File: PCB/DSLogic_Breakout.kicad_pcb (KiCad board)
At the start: 2 copper layers, 24 x 74 mm, 5 parts, among them J1 Interconnect

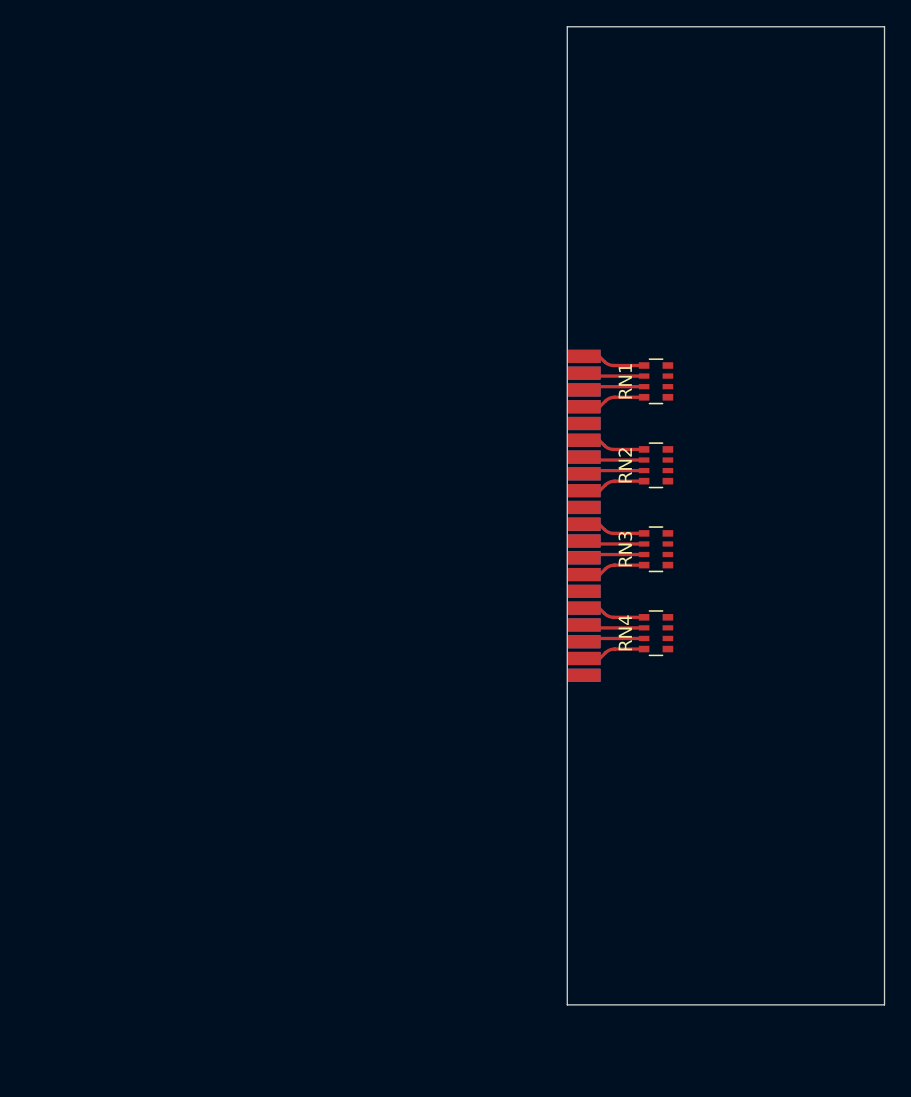
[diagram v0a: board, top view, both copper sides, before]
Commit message: Rev 1 Done
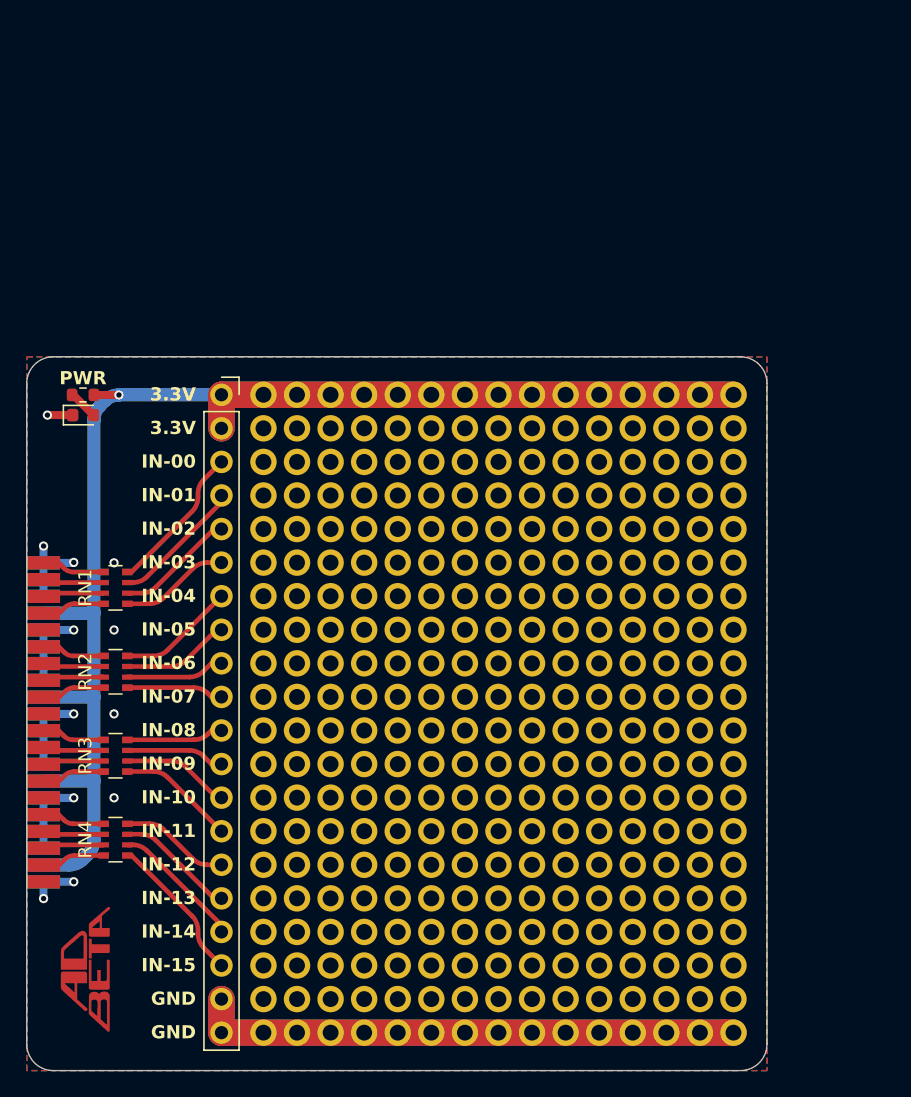
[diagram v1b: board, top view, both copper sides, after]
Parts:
- added ?: , , F.Cu at (141.1, 102.9)
- added ?: , , F.Cu at (123.3, 102.9)
- added ?: , , F.Cu at (125.9, 102.9)
- added ?: , , F.Cu at (133.5, 102.9)
- added ?: , , F.Cu at (141.1, 54.6)
- added ?: , , F.Cu at (133.5, 54.6)
- added ?: , , F.Cu at (151.3, 102.9)
- added ?: , , F.Cu at (146.2, 54.6)
- added ?: , , F.Cu at (156.3, 54.6)
- added ?: , , F.Cu at (138.6, 54.6)
- added ?: , , F.Cu at (136.0, 54.6)
- added ?: , , F.Cu at (151.3, 54.6)
- added ?: , , F.Cu at (123.3, 54.6)
- added ?: , , F.Cu at (146.2, 102.9)
- added ?: , , F.Cu at (148.7, 54.6)
- added ?: , , F.Cu at (153.8, 102.9)
- added ?: , , F.Cu at (130.9, 102.9)
- added ?: , , F.Cu at (130.9, 54.6)
- added ?: , , F.Cu at (120.8, 102.9)
- added ?: , , F.Cu at (128.4, 54.6)
- added ?: , , F.Cu at (156.3, 102.9)
- added ?: , , F.Cu at (128.4, 102.9)
- added ?: , , F.Cu at (148.7, 102.9)
- added ?: , , F.Cu at (143.6, 54.6)
- added ?: , , F.Cu at (153.8, 54.6)
- added ?: , , F.Cu at (138.6, 102.9)
- added ?: , , F.Cu at (143.6, 102.9)
- added ?: , , F.Cu at (136.0, 102.9)
- added ?: , , F.Cu at (125.9, 54.6)
- added D1: PWR, LED_SMD:LED_0603_1608Metric, F.Cu at (107.1, 56.1)
- added J2: Conn_Input, Connector_PinSocket_2.54mm:PinSocket_1x20_P2.54mm_Vertical, F.Cu at (117.6, 54.6)
- added R1: 2K2, Resistor_SMD:R_0603_1608Metric, F.Cu at (107.1, 54.6)
- added REF**: Protoboard_Hole, Footprints:Protoboard_Hole, F.Cu at (125.9, 72.4)
- added REF**: Protoboard_Hole, Footprints:Protoboard_Hole, F.Cu at (156.3, 59.7)
- added REF**: Protoboard_Hole, Footprints:Protoboard_Hole, F.Cu at (128.4, 67.3)
- added REF**: Protoboard_Hole, Footprints:Protoboard_Hole, F.Cu at (125.9, 97.8)
- added REF**: Protoboard_Hole, Footprints:Protoboard_Hole, F.Cu at (128.4, 74.9)
- added REF**: Protoboard_Hole, Footprints:Protoboard_Hole, F.Cu at (156.3, 67.3)
- added REF**: Protoboard_Hole, Footprints:Protoboard_Hole, F.Cu at (141.1, 85.1)
- added REF**: Protoboard_Hole, Footprints:Protoboard_Hole, F.Cu at (133.5, 72.4)
- added REF**: Protoboard_Hole, Footprints:Protoboard_Hole, F.Cu at (141.1, 57.1)
- added REF**: Protoboard_Hole, Footprints:Protoboard_Hole, F.Cu at (123.3, 62.2)
- added REF**: Protoboard_Hole, Footprints:Protoboard_Hole, F.Cu at (141.1, 59.7)
- added REF**: Protoboard_Hole, Footprints:Protoboard_Hole, F.Cu at (128.4, 95.2)
- added REF**: Protoboard_Hole, Footprints:Protoboard_Hole, F.Cu at (146.2, 85.1)
- added REF**: Protoboard_Hole, Footprints:Protoboard_Hole, F.Cu at (156.3, 82.5)
- added REF**: Protoboard_Hole, Footprints:Protoboard_Hole, F.Cu at (120.8, 82.5)
- added REF**: Protoboard_Hole, Footprints:Protoboard_Hole, F.Cu at (148.7, 90.2)
- added REF**: Protoboard_Hole, Footprints:Protoboard_Hole, F.Cu at (146.2, 77.5)
- added REF**: Protoboard_Hole, Footprints:Protoboard_Hole, F.Cu at (151.3, 87.6)
- added REF**: Protoboard_Hole, Footprints:Protoboard_Hole, F.Cu at (151.3, 59.7)
- added REF**: Protoboard_Hole, Footprints:Protoboard_Hole, F.Cu at (143.6, 90.2)
- added REF**: Protoboard_Hole, Footprints:Protoboard_Hole, F.Cu at (153.8, 95.2)
- added REF**: Protoboard_Hole, Footprints:Protoboard_Hole, F.Cu at (138.6, 85.1)
- added REF**: Protoboard_Hole, Footprints:Protoboard_Hole, F.Cu at (125.9, 95.2)
- added REF**: Protoboard_Hole, Footprints:Protoboard_Hole, F.Cu at (125.9, 80.0)
- added REF**: Protoboard_Hole, Footprints:Protoboard_Hole, F.Cu at (143.6, 69.8)
- added REF**: Protoboard_Hole, Footprints:Protoboard_Hole, F.Cu at (123.3, 64.8)
- added REF**: Protoboard_Hole, Footprints:Protoboard_Hole, F.Cu at (128.4, 92.7)
- added REF**: Protoboard_Hole, Footprints:Protoboard_Hole, F.Cu at (156.3, 100.3)
- added REF**: Protoboard_Hole, Footprints:Protoboard_Hole, F.Cu at (136.0, 87.6)
- added REF**: Protoboard_Hole, Footprints:Protoboard_Hole, F.Cu at (123.3, 87.6)
- added REF**: Protoboard_Hole, Footprints:Protoboard_Hole, F.Cu at (156.3, 57.1)
- added REF**: Protoboard_Hole, Footprints:Protoboard_Hole, F.Cu at (156.3, 72.4)
- added REF**: Protoboard_Hole, Footprints:Protoboard_Hole, F.Cu at (151.3, 57.1)
- added REF**: Protoboard_Hole, Footprints:Protoboard_Hole, F.Cu at (133.5, 77.5)
- added REF**: Protoboard_Hole, Footprints:Protoboard_Hole, F.Cu at (153.8, 77.5)
- added REF**: Protoboard_Hole, Footprints:Protoboard_Hole, F.Cu at (120.8, 85.1)
- added REF**: Protoboard_Hole, Footprints:Protoboard_Hole, F.Cu at (123.3, 69.8)
- added REF**: Protoboard_Hole, Footprints:Protoboard_Hole, F.Cu at (146.2, 62.2)
- added REF**: Protoboard_Hole, Footprints:Protoboard_Hole, F.Cu at (128.4, 100.3)
- added REF**: Protoboard_Hole, Footprints:Protoboard_Hole, F.Cu at (151.3, 80.0)
- added REF**: Protoboard_Hole, Footprints:Protoboard_Hole, F.Cu at (130.9, 97.8)
- added REF**: Protoboard_Hole, Footprints:Protoboard_Hole, F.Cu at (130.9, 59.7)
- added REF**: Protoboard_Hole, Footprints:Protoboard_Hole, F.Cu at (130.9, 72.4)
- added REF**: Protoboard_Hole, Footprints:Protoboard_Hole, F.Cu at (141.1, 87.6)
- added REF**: Protoboard_Hole, Footprints:Protoboard_Hole, F.Cu at (120.8, 87.6)
- added REF**: Protoboard_Hole, Footprints:Protoboard_Hole, F.Cu at (141.1, 69.8)
- added REF**: Protoboard_Hole, Footprints:Protoboard_Hole, F.Cu at (148.7, 97.8)
- added REF**: Protoboard_Hole, Footprints:Protoboard_Hole, F.Cu at (130.9, 62.2)
- added REF**: Protoboard_Hole, Footprints:Protoboard_Hole, F.Cu at (141.1, 62.2)
- added REF**: Protoboard_Hole, Footprints:Protoboard_Hole, F.Cu at (133.5, 59.7)
- added REF**: Protoboard_Hole, Footprints:Protoboard_Hole, F.Cu at (138.6, 69.8)
- added REF**: Protoboard_Hole, Footprints:Protoboard_Hole, F.Cu at (130.9, 92.7)
- added REF**: Protoboard_Hole, Footprints:Protoboard_Hole, F.Cu at (148.7, 77.5)
- added REF**: Protoboard_Hole, Footprints:Protoboard_Hole, F.Cu at (125.9, 69.8)
- added REF**: Protoboard_Hole, Footprints:Protoboard_Hole, F.Cu at (120.8, 67.3)
- added REF**: Protoboard_Hole, Footprints:Protoboard_Hole, F.Cu at (120.8, 72.4)
- added REF**: Protoboard_Hole, Footprints:Protoboard_Hole, F.Cu at (156.3, 92.7)
- added REF**: Protoboard_Hole, Footprints:Protoboard_Hole, F.Cu at (148.7, 82.5)
- added REF**: Protoboard_Hole, Footprints:Protoboard_Hole, F.Cu at (133.5, 100.3)
- added REF**: Protoboard_Hole, Footprints:Protoboard_Hole, F.Cu at (120.8, 62.2)
- added REF**: Protoboard_Hole, Footprints:Protoboard_Hole, F.Cu at (148.7, 57.1)
- added REF**: Protoboard_Hole, Footprints:Protoboard_Hole, F.Cu at (153.8, 82.5)
- added REF**: Protoboard_Hole, Footprints:Protoboard_Hole, F.Cu at (153.8, 87.6)
- added REF**: Protoboard_Hole, Footprints:Protoboard_Hole, F.Cu at (125.9, 62.2)
- added REF**: Protoboard_Hole, Footprints:Protoboard_Hole, F.Cu at (120.8, 95.2)
- added REF**: Protoboard_Hole, Footprints:Protoboard_Hole, F.Cu at (136.0, 64.8)
- added REF**: Protoboard_Hole, Footprints:Protoboard_Hole, F.Cu at (130.9, 100.3)
- added REF**: Protoboard_Hole, Footprints:Protoboard_Hole, F.Cu at (130.9, 69.8)
- added REF**: Protoboard_Hole, Footprints:Protoboard_Hole, F.Cu at (123.3, 59.7)
- added REF**: Protoboard_Hole, Footprints:Protoboard_Hole, F.Cu at (128.4, 87.6)
- added REF**: Protoboard_Hole, Footprints:Protoboard_Hole, F.Cu at (148.7, 85.1)
- added REF**: Protoboard_Hole, Footprints:Protoboard_Hole, F.Cu at (143.6, 87.6)
- added REF**: Protoboard_Hole, Footprints:Protoboard_Hole, F.Cu at (148.7, 92.7)
- added REF**: Protoboard_Hole, Footprints:Protoboard_Hole, F.Cu at (123.3, 57.1)
- added REF**: Protoboard_Hole, Footprints:Protoboard_Hole, F.Cu at (153.8, 72.4)
- added REF**: Protoboard_Hole, Footprints:Protoboard_Hole, F.Cu at (130.9, 80.0)
- added REF**: Protoboard_Hole, Footprints:Protoboard_Hole, F.Cu at (123.3, 77.5)
- added REF**: Protoboard_Hole, Footprints:Protoboard_Hole, F.Cu at (141.1, 77.5)
- added REF**: Protoboard_Hole, Footprints:Protoboard_Hole, F.Cu at (146.2, 82.5)
- added REF**: Protoboard_Hole, Footprints:Protoboard_Hole, F.Cu at (153.8, 80.0)
- added REF**: Protoboard_Hole, Footprints:Protoboard_Hole, F.Cu at (146.2, 87.6)
- added REF**: Protoboard_Hole, Footprints:Protoboard_Hole, F.Cu at (153.8, 69.8)
- added REF**: Protoboard_Hole, Footprints:Protoboard_Hole, F.Cu at (136.0, 57.1)
- added REF**: Protoboard_Hole, Footprints:Protoboard_Hole, F.Cu at (143.6, 72.4)
- added REF**: Protoboard_Hole, Footprints:Protoboard_Hole, F.Cu at (123.3, 72.4)
- added REF**: Protoboard_Hole, Footprints:Protoboard_Hole, F.Cu at (146.2, 74.9)
- added REF**: Protoboard_Hole, Footprints:Protoboard_Hole, F.Cu at (120.8, 74.9)
- added REF**: Protoboard_Hole, Footprints:Protoboard_Hole, F.Cu at (128.4, 97.8)
- added REF**: Protoboard_Hole, Footprints:Protoboard_Hole, F.Cu at (136.0, 92.7)
- added REF**: Protoboard_Hole, Footprints:Protoboard_Hole, F.Cu at (153.8, 57.1)
- added REF**: Protoboard_Hole, Footprints:Protoboard_Hole, F.Cu at (136.0, 95.2)
- added REF**: Protoboard_Hole, Footprints:Protoboard_Hole, F.Cu at (156.3, 90.2)
- added REF**: Protoboard_Hole, Footprints:Protoboard_Hole, F.Cu at (125.9, 67.3)
- added REF**: Protoboard_Hole, Footprints:Protoboard_Hole, F.Cu at (125.9, 82.5)
- added REF**: Protoboard_Hole, Footprints:Protoboard_Hole, F.Cu at (141.1, 82.5)
- added REF**: Protoboard_Hole, Footprints:Protoboard_Hole, F.Cu at (151.3, 72.4)
- added REF**: Protoboard_Hole, Footprints:Protoboard_Hole, F.Cu at (151.3, 67.3)
- added REF**: Protoboard_Hole, Footprints:Protoboard_Hole, F.Cu at (156.3, 74.9)
- added REF**: Protoboard_Hole, Footprints:Protoboard_Hole, F.Cu at (151.3, 85.1)
- added REF**: Protoboard_Hole, Footprints:Protoboard_Hole, F.Cu at (133.5, 57.1)
- added REF**: Protoboard_Hole, Footprints:Protoboard_Hole, F.Cu at (156.3, 80.0)
- added REF**: Protoboard_Hole, Footprints:Protoboard_Hole, F.Cu at (128.4, 80.0)
- added REF**: Protoboard_Hole, Footprints:Protoboard_Hole, F.Cu at (128.4, 57.1)
- added REF**: Protoboard_Hole, Footprints:Protoboard_Hole, F.Cu at (123.3, 90.2)
- added REF**: Protoboard_Hole, Footprints:Protoboard_Hole, F.Cu at (148.7, 87.6)
- added REF**: Protoboard_Hole, Footprints:Protoboard_Hole, F.Cu at (120.8, 64.8)
- added REF**: Protoboard_Hole, Footprints:Protoboard_Hole, F.Cu at (148.7, 100.3)
- added REF**: Protoboard_Hole, Footprints:Protoboard_Hole, F.Cu at (153.8, 97.8)
- added REF**: Protoboard_Hole, Footprints:Protoboard_Hole, F.Cu at (143.6, 100.3)
- added REF**: Protoboard_Hole, Footprints:Protoboard_Hole, F.Cu at (146.2, 57.1)
- added REF**: Protoboard_Hole, Footprints:Protoboard_Hole, F.Cu at (148.7, 67.3)
- added REF**: Protoboard_Hole, Footprints:Protoboard_Hole, F.Cu at (123.3, 92.7)
- added REF**: Protoboard_Hole, Footprints:Protoboard_Hole, F.Cu at (125.9, 85.1)
- added REF**: Protoboard_Hole, Footprints:Protoboard_Hole, F.Cu at (153.8, 64.8)
- added REF**: Protoboard_Hole, Footprints:Protoboard_Hole, F.Cu at (151.3, 69.8)
- added REF**: Protoboard_Hole, Footprints:Protoboard_Hole, F.Cu at (143.6, 97.8)
- added REF**: Protoboard_Hole, Footprints:Protoboard_Hole, F.Cu at (138.6, 72.4)
- added REF**: Protoboard_Hole, Footprints:Protoboard_Hole, F.Cu at (136.0, 97.8)
- added REF**: Protoboard_Hole, Footprints:Protoboard_Hole, F.Cu at (151.3, 74.9)
- added REF**: Protoboard_Hole, Footprints:Protoboard_Hole, F.Cu at (143.6, 82.5)
- added REF**: Protoboard_Hole, Footprints:Protoboard_Hole, F.Cu at (143.6, 80.0)
- added REF**: Protoboard_Hole, Footprints:Protoboard_Hole, F.Cu at (130.9, 74.9)
- added REF**: Protoboard_Hole, Footprints:Protoboard_Hole, F.Cu at (141.1, 95.2)
- added REF**: Protoboard_Hole, Footprints:Protoboard_Hole, F.Cu at (143.6, 59.7)
- added REF**: Protoboard_Hole, Footprints:Protoboard_Hole, F.Cu at (136.0, 82.5)
- added REF**: Protoboard_Hole, Footprints:Protoboard_Hole, F.Cu at (148.7, 74.9)
- added REF**: Protoboard_Hole, Footprints:Protoboard_Hole, F.Cu at (123.3, 74.9)
- added REF**: Protoboard_Hole, Footprints:Protoboard_Hole, F.Cu at (146.2, 90.2)
- added REF**: Protoboard_Hole, Footprints:Protoboard_Hole, F.Cu at (120.8, 97.8)
- added REF**: Protoboard_Hole, Footprints:Protoboard_Hole, F.Cu at (156.3, 85.1)
- added REF**: Protoboard_Hole, Footprints:Protoboard_Hole, F.Cu at (138.6, 90.2)
- added REF**: Protoboard_Hole, Footprints:Protoboard_Hole, F.Cu at (136.0, 74.9)
- added REF**: Protoboard_Hole, Footprints:Protoboard_Hole, F.Cu at (130.9, 82.5)
- added REF**: Protoboard_Hole, Footprints:Protoboard_Hole, F.Cu at (151.3, 97.8)
- added REF**: Protoboard_Hole, Footprints:Protoboard_Hole, F.Cu at (146.2, 100.3)
- added REF**: Protoboard_Hole, Footprints:Protoboard_Hole, F.Cu at (136.0, 72.4)
- added REF**: Protoboard_Hole, Footprints:Protoboard_Hole, F.Cu at (128.4, 82.5)
- added REF**: Protoboard_Hole, Footprints:Protoboard_Hole, F.Cu at (125.9, 100.3)
- added REF**: Protoboard_Hole, Footprints:Protoboard_Hole, F.Cu at (141.1, 74.9)
- added REF**: Protoboard_Hole, Footprints:Protoboard_Hole, F.Cu at (151.3, 82.5)
- added REF**: Protoboard_Hole, Footprints:Protoboard_Hole, F.Cu at (138.6, 80.0)
- added REF**: Protoboard_Hole, Footprints:Protoboard_Hole, F.Cu at (146.2, 72.4)
- added REF**: Protoboard_Hole, Footprints:Protoboard_Hole, F.Cu at (146.2, 59.7)
- added REF**: Protoboard_Hole, Footprints:Protoboard_Hole, F.Cu at (138.6, 97.8)
- added REF**: Protoboard_Hole, Footprints:Protoboard_Hole, F.Cu at (138.6, 74.9)
- added REF**: Protoboard_Hole, Footprints:Protoboard_Hole, F.Cu at (130.9, 87.6)
- added REF**: Protoboard_Hole, Footprints:Protoboard_Hole, F.Cu at (133.5, 92.7)
- added REF**: Protoboard_Hole, Footprints:Protoboard_Hole, F.Cu at (141.1, 90.2)
- added REF**: Protoboard_Hole, Footprints:Protoboard_Hole, F.Cu at (156.3, 62.2)
- added REF**: Protoboard_Hole, Footprints:Protoboard_Hole, F.Cu at (138.6, 77.5)
- added REF**: Protoboard_Hole, Footprints:Protoboard_Hole, F.Cu at (130.9, 64.8)
- added REF**: Protoboard_Hole, Footprints:Protoboard_Hole, F.Cu at (146.2, 95.2)
- added REF**: Protoboard_Hole, Footprints:Protoboard_Hole, F.Cu at (128.4, 90.2)
- added REF**: Protoboard_Hole, Footprints:Protoboard_Hole, F.Cu at (136.0, 62.2)
- added REF**: Protoboard_Hole, Footprints:Protoboard_Hole, F.Cu at (133.5, 95.2)
- added REF**: Protoboard_Hole, Footprints:Protoboard_Hole, F.Cu at (120.8, 80.0)
- added REF**: Protoboard_Hole, Footprints:Protoboard_Hole, F.Cu at (125.9, 64.8)
- added REF**: Protoboard_Hole, Footprints:Protoboard_Hole, F.Cu at (120.8, 90.2)
- added REF**: Protoboard_Hole, Footprints:Protoboard_Hole, F.Cu at (136.0, 69.8)
- added REF**: Protoboard_Hole, Footprints:Protoboard_Hole, F.Cu at (156.3, 87.6)
- added REF**: Protoboard_Hole, Footprints:Protoboard_Hole, F.Cu at (120.8, 100.3)
- added REF**: Protoboard_Hole, Footprints:Protoboard_Hole, F.Cu at (151.3, 95.2)
- added REF**: Protoboard_Hole, Footprints:Protoboard_Hole, F.Cu at (141.1, 97.8)
- added REF**: Protoboard_Hole, Footprints:Protoboard_Hole, F.Cu at (130.9, 90.2)
- added REF**: Protoboard_Hole, Footprints:Protoboard_Hole, F.Cu at (148.7, 80.0)
- added REF**: Protoboard_Hole, Footprints:Protoboard_Hole, F.Cu at (130.9, 77.5)
- added REF**: Protoboard_Hole, Footprints:Protoboard_Hole, F.Cu at (156.3, 95.2)
- added REF**: Protoboard_Hole, Footprints:Protoboard_Hole, F.Cu at (138.6, 95.2)
- added REF**: Protoboard_Hole, Footprints:Protoboard_Hole, F.Cu at (143.6, 57.1)
- added REF**: Protoboard_Hole, Footprints:Protoboard_Hole, F.Cu at (130.9, 95.2)
- added REF**: Protoboard_Hole, Footprints:Protoboard_Hole, F.Cu at (141.1, 67.3)
- added REF**: Protoboard_Hole, Footprints:Protoboard_Hole, F.Cu at (133.5, 74.9)
- added REF**: Protoboard_Hole, Footprints:Protoboard_Hole, F.Cu at (148.7, 59.7)
- added REF**: Protoboard_Hole, Footprints:Protoboard_Hole, F.Cu at (125.9, 59.7)
- added REF**: Protoboard_Hole, Footprints:Protoboard_Hole, F.Cu at (138.6, 92.7)
- added REF**: Protoboard_Hole, Footprints:Protoboard_Hole, F.Cu at (136.0, 90.2)
- added REF**: Protoboard_Hole, Footprints:Protoboard_Hole, F.Cu at (138.6, 82.5)
- added REF**: Protoboard_Hole, Footprints:Protoboard_Hole, F.Cu at (148.7, 64.8)
- added REF**: Protoboard_Hole, Footprints:Protoboard_Hole, F.Cu at (153.8, 62.2)
- added REF**: Protoboard_Hole, Footprints:Protoboard_Hole, F.Cu at (138.6, 57.1)
- added REF**: Protoboard_Hole, Footprints:Protoboard_Hole, F.Cu at (153.8, 67.3)
- added REF**: Protoboard_Hole, Footprints:Protoboard_Hole, F.Cu at (138.6, 100.3)
- added REF**: Protoboard_Hole, Footprints:Protoboard_Hole, F.Cu at (138.6, 62.2)
- added REF**: Protoboard_Hole, Footprints:Protoboard_Hole, F.Cu at (133.5, 80.0)
- added REF**: Protoboard_Hole, Footprints:Protoboard_Hole, F.Cu at (125.9, 74.9)
- added REF**: Protoboard_Hole, Footprints:Protoboard_Hole, F.Cu at (146.2, 92.7)
- added REF**: Protoboard_Hole, Footprints:Protoboard_Hole, F.Cu at (153.8, 59.7)
- added REF**: Protoboard_Hole, Footprints:Protoboard_Hole, F.Cu at (133.5, 67.3)
- added REF**: Protoboard_Hole, Footprints:Protoboard_Hole, F.Cu at (128.4, 85.1)
- added REF**: Protoboard_Hole, Footprints:Protoboard_Hole, F.Cu at (146.2, 67.3)
- added REF**: Protoboard_Hole, Footprints:Protoboard_Hole, F.Cu at (123.3, 97.8)
- added REF**: Protoboard_Hole, Footprints:Protoboard_Hole, F.Cu at (133.5, 62.2)
- added REF**: Protoboard_Hole, Footprints:Protoboard_Hole, F.Cu at (133.5, 69.8)
- added REF**: Protoboard_Hole, Footprints:Protoboard_Hole, F.Cu at (151.3, 100.3)
- added REF**: Protoboard_Hole, Footprints:Protoboard_Hole, F.Cu at (143.6, 95.2)
- added REF**: Protoboard_Hole, Footprints:Protoboard_Hole, F.Cu at (136.0, 85.1)
- added REF**: Protoboard_Hole, Footprints:Protoboard_Hole, F.Cu at (141.1, 92.7)
- added REF**: Protoboard_Hole, Footprints:Protoboard_Hole, F.Cu at (138.6, 59.7)
- added REF**: Protoboard_Hole, Footprints:Protoboard_Hole, F.Cu at (153.8, 74.9)
- added REF**: Protoboard_Hole, Footprints:Protoboard_Hole, F.Cu at (141.1, 72.4)
- added REF**: Protoboard_Hole, Footprints:Protoboard_Hole, F.Cu at (151.3, 62.2)
- added REF**: Protoboard_Hole, Footprints:Protoboard_Hole, F.Cu at (123.3, 85.1)
- added REF**: Protoboard_Hole, Footprints:Protoboard_Hole, F.Cu at (156.3, 77.5)
- added REF**: Protoboard_Hole, Footprints:Protoboard_Hole, F.Cu at (143.6, 77.5)
- added REF**: Protoboard_Hole, Footprints:Protoboard_Hole, F.Cu at (123.3, 95.2)
- added REF**: Protoboard_Hole, Footprints:Protoboard_Hole, F.Cu at (133.5, 90.2)
- added REF**: Protoboard_Hole, Footprints:Protoboard_Hole, F.Cu at (146.2, 69.8)
- added REF**: Protoboard_Hole, Footprints:Protoboard_Hole, F.Cu at (128.4, 72.4)
- added REF**: Protoboard_Hole, Footprints:Protoboard_Hole, F.Cu at (125.9, 77.5)
- added REF**: Protoboard_Hole, Footprints:Protoboard_Hole, F.Cu at (133.5, 85.1)
- added REF**: Protoboard_Hole, Footprints:Protoboard_Hole, F.Cu at (151.3, 90.2)
- added REF**: Protoboard_Hole, Footprints:Protoboard_Hole, F.Cu at (148.7, 95.2)
- added REF**: Protoboard_Hole, Footprints:Protoboard_Hole, F.Cu at (143.6, 67.3)
- added REF**: Protoboard_Hole, Footprints:Protoboard_Hole, F.Cu at (143.6, 62.2)
- added REF**: Protoboard_Hole, Footprints:Protoboard_Hole, F.Cu at (123.3, 80.0)
- added REF**: Protoboard_Hole, Footprints:Protoboard_Hole, F.Cu at (138.6, 64.8)
- added REF**: Protoboard_Hole, Footprints:Protoboard_Hole, F.Cu at (120.8, 54.6)
- added REF**: Protoboard_Hole, Footprints:Protoboard_Hole, F.Cu at (125.9, 92.7)
- added REF**: Protoboard_Hole, Footprints:Protoboard_Hole, F.Cu at (133.5, 64.8)
- added REF**: Protoboard_Hole, Footprints:Protoboard_Hole, F.Cu at (120.8, 59.7)
- added REF**: Protoboard_Hole, Footprints:Protoboard_Hole, F.Cu at (125.9, 87.6)
- added REF**: Protoboard_Hole, Footprints:Protoboard_Hole, F.Cu at (123.3, 100.3)
- added REF**: Protoboard_Hole, Footprints:Protoboard_Hole, F.Cu at (130.9, 85.1)
- added REF**: Protoboard_Hole, Footprints:Protoboard_Hole, F.Cu at (136.0, 77.5)
- added REF**: Protoboard_Hole, Footprints:Protoboard_Hole, F.Cu at (146.2, 64.8)
- added REF**: Protoboard_Hole, Footprints:Protoboard_Hole, F.Cu at (125.9, 57.1)
- added REF**: Protoboard_Hole, Footprints:Protoboard_Hole, F.Cu at (138.6, 87.6)
- added REF**: Protoboard_Hole, Footprints:Protoboard_Hole, F.Cu at (125.9, 90.2)
- added REF**: Protoboard_Hole, Footprints:Protoboard_Hole, F.Cu at (128.4, 62.2)
- added REF**: Protoboard_Hole, Footprints:Protoboard_Hole, F.Cu at (120.8, 92.7)
- added REF**: Protoboard_Hole, Footprints:Protoboard_Hole, F.Cu at (130.9, 67.3)
- added REF**: Protoboard_Hole, Footprints:Protoboard_Hole, F.Cu at (133.5, 97.8)
- added REF**: Protoboard_Hole, Footprints:Protoboard_Hole, F.Cu at (156.3, 64.8)
- added REF**: Protoboard_Hole, Footprints:Protoboard_Hole, F.Cu at (128.4, 77.5)
- added REF**: Protoboard_Hole, Footprints:Protoboard_Hole, F.Cu at (136.0, 100.3)
- added REF**: Protoboard_Hole, Footprints:Protoboard_Hole, F.Cu at (138.6, 67.3)
- added REF**: Protoboard_Hole, Footprints:Protoboard_Hole, F.Cu at (120.8, 57.1)
- added REF**: Protoboard_Hole, Footprints:Protoboard_Hole, F.Cu at (123.3, 67.3)
- added REF**: Protoboard_Hole, Footprints:Protoboard_Hole, F.Cu at (148.7, 69.8)
- added REF**: Protoboard_Hole, Footprints:Protoboard_Hole, F.Cu at (153.8, 100.3)
- added REF**: Protoboard_Hole, Footprints:Protoboard_Hole, F.Cu at (120.8, 77.5)
- added REF**: Protoboard_Hole, Footprints:Protoboard_Hole, F.Cu at (151.3, 64.8)
- added REF**: Protoboard_Hole, Footprints:Protoboard_Hole, F.Cu at (151.3, 92.7)
- added REF**: Protoboard_Hole, Footprints:Protoboard_Hole, F.Cu at (153.8, 90.2)
- added REF**: Protoboard_Hole, Footprints:Protoboard_Hole, F.Cu at (156.3, 97.8)
- added REF**: Protoboard_Hole, Footprints:Protoboard_Hole, F.Cu at (143.6, 64.8)
- added REF**: Protoboard_Hole, Footprints:Protoboard_Hole, F.Cu at (153.8, 92.7)
- added REF**: Protoboard_Hole, Footprints:Protoboard_Hole, F.Cu at (136.0, 59.7)
- added REF**: Protoboard_Hole, Footprints:Protoboard_Hole, F.Cu at (120.8, 69.8)
- added REF**: Protoboard_Hole, Footprints:Protoboard_Hole, F.Cu at (133.5, 82.5)
- added REF**: Protoboard_Hole, Footprints:Protoboard_Hole, F.Cu at (148.7, 72.4)
- added REF**: Protoboard_Hole, Footprints:Protoboard_Hole, F.Cu at (133.5, 87.6)
- added REF**: Protoboard_Hole, Footprints:Protoboard_Hole, F.Cu at (141.1, 80.0)
- added REF**: Protoboard_Hole, Footprints:Protoboard_Hole, F.Cu at (136.0, 67.3)
- added REF**: Protoboard_Hole, Footprints:Protoboard_Hole, F.Cu at (148.7, 62.2)
- added REF**: Protoboard_Hole, Footprints:Protoboard_Hole, F.Cu at (123.3, 82.5)
- added REF**: Protoboard_Hole, Footprints:Protoboard_Hole, F.Cu at (143.6, 74.9)
- added REF**: Protoboard_Hole, Footprints:Protoboard_Hole, F.Cu at (156.3, 69.8)
- added REF**: Protoboard_Hole, Footprints:Protoboard_Hole, F.Cu at (146.2, 80.0)
- added REF**: Protoboard_Hole, Footprints:Protoboard_Hole, F.Cu at (153.8, 85.1)
- added REF**: Protoboard_Hole, Footprints:Protoboard_Hole, F.Cu at (128.4, 64.8)
- added REF**: Protoboard_Hole, Footprints:Protoboard_Hole, F.Cu at (136.0, 80.0)
- added REF**: Protoboard_Hole, Footprints:Protoboard_Hole, F.Cu at (141.1, 100.3)
- added REF**: Protoboard_Hole, Footprints:Protoboard_Hole, F.Cu at (128.4, 69.8)
- added REF**: Protoboard_Hole, Footprints:Protoboard_Hole, F.Cu at (143.6, 85.1)
- added REF**: Protoboard_Hole, Footprints:Protoboard_Hole, F.Cu at (141.1, 64.8)
- added REF**: Protoboard_Hole, Footprints:Protoboard_Hole, F.Cu at (130.9, 57.1)
- added REF**: Protoboard_Hole, Footprints:Protoboard_Hole, F.Cu at (146.2, 97.8)
- added REF**: Protoboard_Hole, Footprints:Protoboard_Hole, F.Cu at (143.6, 92.7)
- added REF**: Protoboard_Hole, Footprints:Protoboard_Hole, F.Cu at (128.4, 59.7)
- added REF**: Protoboard_Hole, Footprints:Protoboard_Hole, F.Cu at (151.3, 77.5)
- moved RN1 43.8 mm to (109.6, 69.2)
- moved RN2 43.8 mm to (109.6, 75.6)
- moved RN3 43.8 mm to (109.6, 81.9)
- moved RN4 43.8 mm to (109.6, 88.3)
- moved J1 43.8 mm to (104.1, 79.4)
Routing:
- net +3.3V: track 0.00 -> 143.1 mm, vias 0 -> 1
- net GND: track 0.00 -> 112.4 mm, vias 0 -> 12
- net /INPUT_00: track 0.00 -> 11.3 mm
- net /INPUT_15: track 0.00 -> 11.3 mm
- net /INPUT_14: track 0.00 -> 10.1 mm
- net /INPUT_01: track 0.00 -> 10.1 mm
- net /INPUT_02: track 0.00 -> 9.06 mm
- net /INPUT_13: track 0.00 -> 9.06 mm
- net /INPUT_04: track 0.00 -> 8.92 mm
- net /INPUT_11: track 0.00 -> 8.92 mm
- net /INPUT_12: track 0.00 -> 8.26 mm
- net /INPUT_03: track 0.00 -> 8.26 mm
- net /INPUT_10: track 0.00 -> 8.20 mm
- net /INPUT_05: track 0.00 -> 8.20 mm
- net /INPUT_09: track 0.00 -> 7.48 mm
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- added copper zone on B.Cu, net GND
- added copper zone on F.Cu, net GND
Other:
- board size 24 x 74 mm -> 56 x 54 mm
- board text added: "3.3V"
- board text added: "GND"
- board text added: "IN-00"
- board text added: "IN-01"
- board text added: "IN-02"
- board text added: "IN-03"
- board text added: "IN-04"
- board text added: "IN-05"
- board text added: "IN-06"
- board text added: "IN-07"
- board text added: "IN-08"
- board text added: "IN-09"
- board text added: "IN-10"
- board text added: "IN-11"
- board text added: "IN-12"
- board text added: "IN-13"
- board text added: "IN-14"
- board text added: "IN-15"
- board text added: "PWR"
- board text removed: "PCB Max Height: 74mm"
